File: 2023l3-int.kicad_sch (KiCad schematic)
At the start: 8 parts, among them J1 0526101433, J2 52610-0833

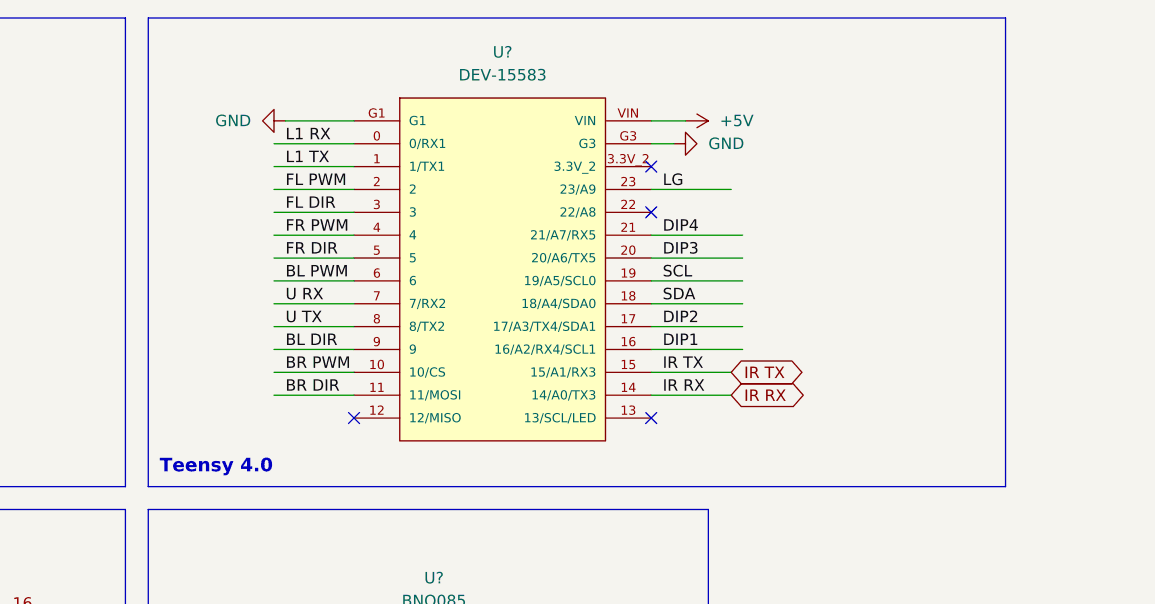
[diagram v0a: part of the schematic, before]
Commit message: 3d pcb
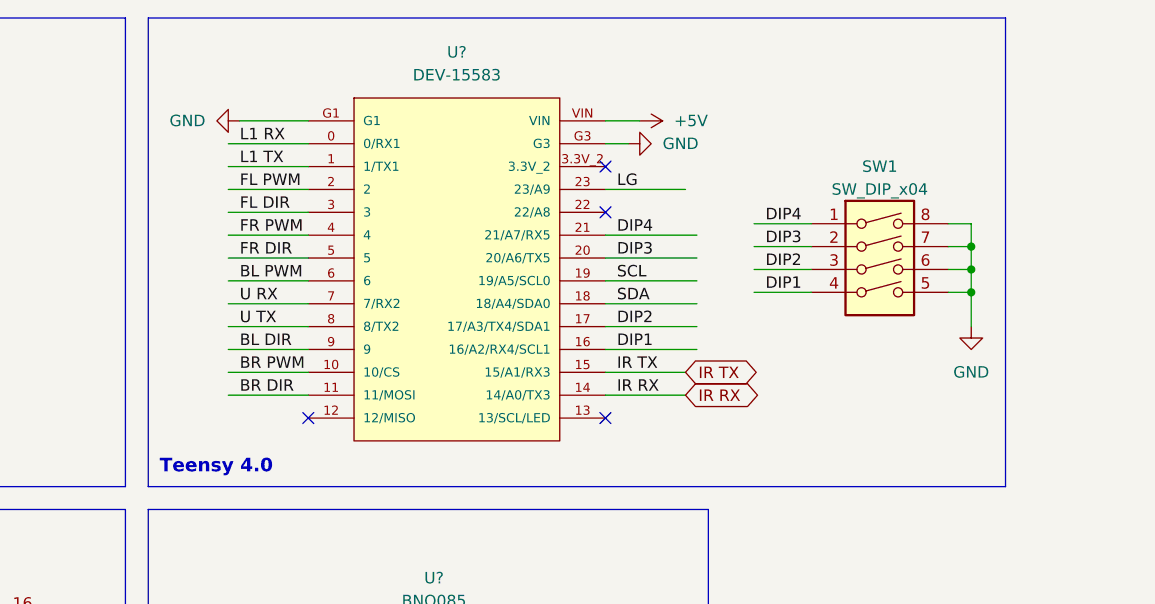
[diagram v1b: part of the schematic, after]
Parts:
- added SW1: SW_DIP_x04, Button_Switch_SMD:SW_DIP_SPSTx04_Slide_6.7x11.72mm_W8.61mm_P2.54mm_LowProfile, symbol Switch:SW_DIP_x04
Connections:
- net DIP1: now also SW1.4
- net DIP2: now also SW1.3
- net DIP3: now also SW1.2
- net DIP4: now also SW1.1
- net GND: now also SW1.5, SW1.6, SW1.7, SW1.8
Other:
- moved on the sheet: U?
